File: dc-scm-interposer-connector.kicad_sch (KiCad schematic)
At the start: 2 parts, among them J2001 PinSocket_2x10_P2.54mm_SMD, J2002 PinSocket_2x10_P2.54mm_SMD

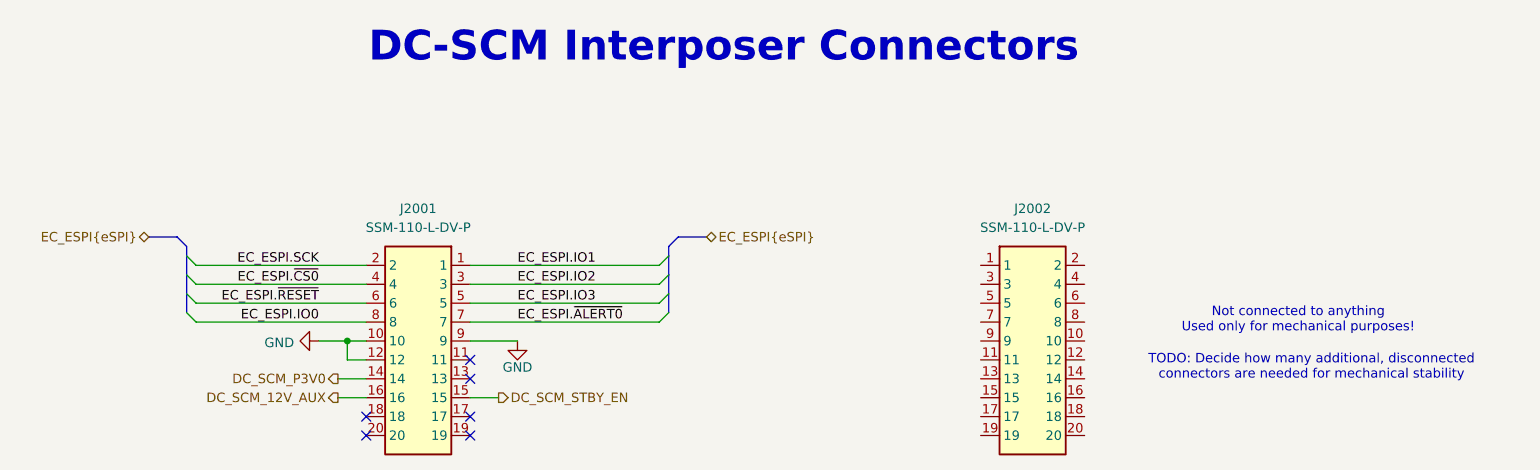
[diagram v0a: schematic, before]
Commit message: [#103224] Initial placement/visualization
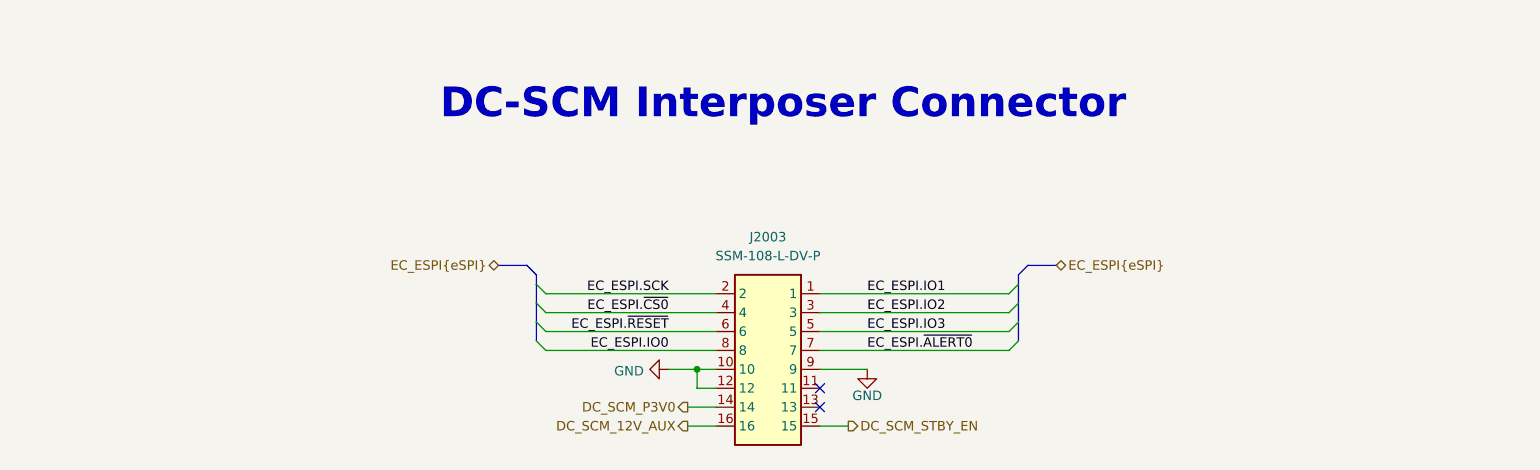
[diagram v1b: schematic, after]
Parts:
- removed J2001, J2002: PinSocket_2x10_P2.54mm_SMD, antmicro-footprints:PinSocket_2x10_P2.54mm_SMD, symbol Antmicro Symbols:PinSocket_2x10_P2.54mm_SMD
- added J2003: PinSocket_2x8_P2.54mm_SMD, antmicro-footprints:PinSocket_2x8_P2.54mm_SMD, symbol Antmicro Symbols:PinSocket_2x8_P2.54mm_SMD
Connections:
- net DC_SCM_12V_AUX: now also J2003.16
- net DC_SCM_P3V0: now also J2003.14
- net DC_SCM_STBY_EN: now also J2003.15
- net EC_ESPI.IO0: now also J2003.8
- net EC_ESPI.IO1: now also J2003.1
- net EC_ESPI.IO2: now also J2003.3
- net EC_ESPI.IO3: now also J2003.5
- net EC_ESPI.SCK: now also J2003.2
- net EC_ESPI.~{ALERT0}: now also J2003.7
- net EC_ESPI.~{CS0}: now also J2003.4
- net EC_ESPI.~{RESET}: now also J2003.6
- net GND: now also J2003.10, J2003.12, J2003.9
- no-connect marks 6 -> 2
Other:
- note added: "DC-SCM Interposer Connector"
- note removed: "DC-SCM Interposer Connectors"
- note removed: "Not connected to anything Used only for mechanical purposes!"
- note removed: "TODO: Decide how many additional, disconnected connectors are needed for mechanical stability"
